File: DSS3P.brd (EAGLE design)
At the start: 399.7 x 251.8 mm, 299 parts, among them J1 J7MM

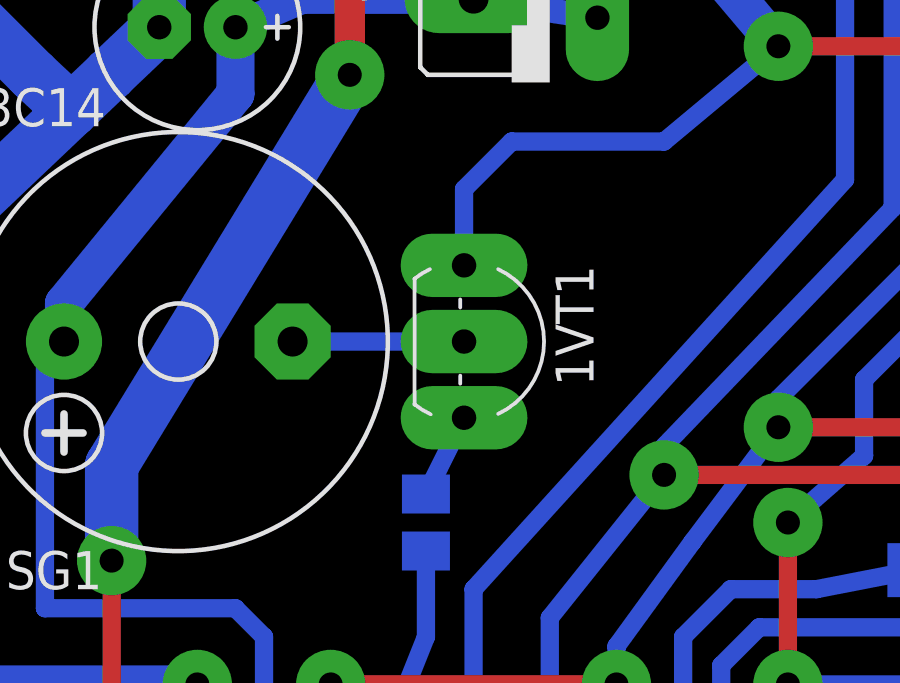
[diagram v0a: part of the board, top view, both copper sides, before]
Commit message: +epf
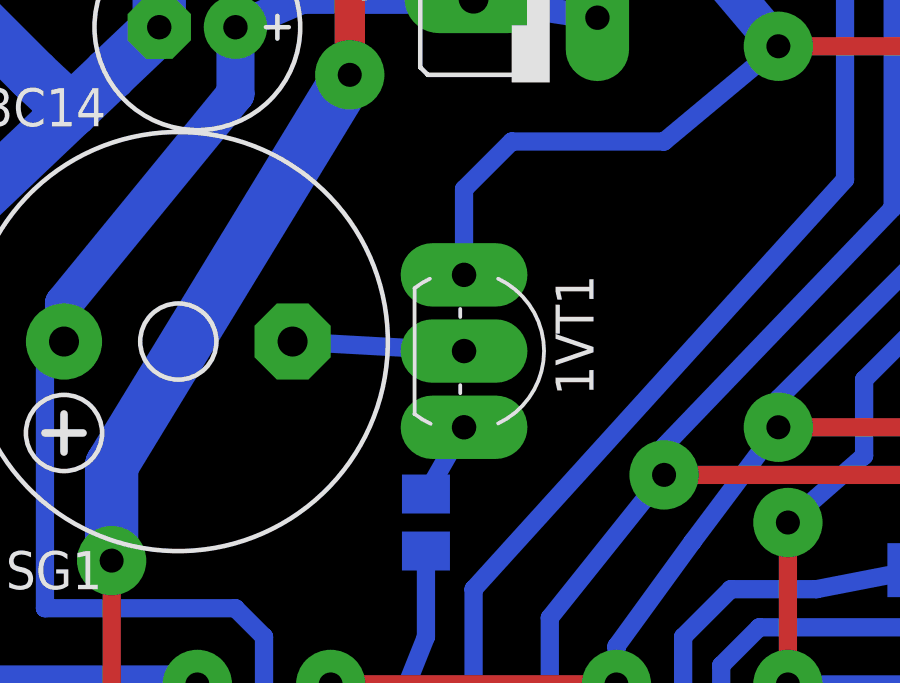
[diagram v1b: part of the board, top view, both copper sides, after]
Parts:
- moved 1VT1 0.32 mm to (127.3, 152.7)
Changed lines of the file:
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@@
 </element>
 <element name="1R31" library="resistor" package="0207/10" value="33k" x="136.525" y="132.715" rot="R270"/>
-<element name="1VT1" library="transistor" package="TO92-ECB" value="" x="127.3175" y="153.035" rot="R270"/>
+<element name="1VT1" library="transistor" package="TO92-ECB" value="" x="127.3175" y="152.7175" rot="R270"/>
 <element name="SG1" library="buzzer" package="F/CM12P" value="F/CM12P" x="117.7925" y="153.035" rot="R180">
 <attribute name="OC_NEWARK" value="unknown" x="-47.307496875" y="215.265003125" size="1.778" layer="27" rot="R180" display="off"/>
@@
 <wire x1="152.7175" y1="137.795" x2="154.94" y2="137.795" width="1.27" layer="16"/>
 <wire x1="154.94" y1="125.73" x2="153.3525" y2="124.46" width="1.27" layer="16"/>
-<wire x1="127.3175" y1="155.575" x2="127.3175" y2="158.115" width="0.6096" layer="16"/>
+<wire x1="127.3175" y1="155.2575" x2="127.3175" y2="158.115" width="0.6096" layer="16"/>
 <wire x1="127.3175" y1="158.115" x2="128.905" y2="159.7025" width="0.6096" layer="16"/>
 <wire x1="128.905" y1="159.7025" x2="133.985" y2="159.7025" width="0.6096" layer="16"/>
@@
 <contactref element="1VT1" pad="B"/>
 <contactref element="1R32" pad="1"/>
-<wire x1="126.0475" y1="147.9525" x2="127.3175" y2="150.495" width="0.6096" layer="16"/>
+<wire x1="126.0475" y1="147.9525" x2="127.3175" y2="150.1775" width="0.6096" layer="16"/>
 </signal>
 <signal name="V_PROG">
@@
 <contactref element="1VT1" pad="C"/>
 <contactref element="SG1" pad="-"/>
-<wire x1="121.6025" y1="153.035" x2="127.3175" y2="153.035" width="0.6096" layer="16"/>
+<wire x1="121.6025" y1="153.035" x2="127.3175" y2="152.7175" width="0.6096" layer="16"/>
 </signal>
 <signal name="N$14">
